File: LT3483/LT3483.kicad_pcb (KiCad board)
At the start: 2 copper layers, 19.8 x 40.1 mm, 15 parts

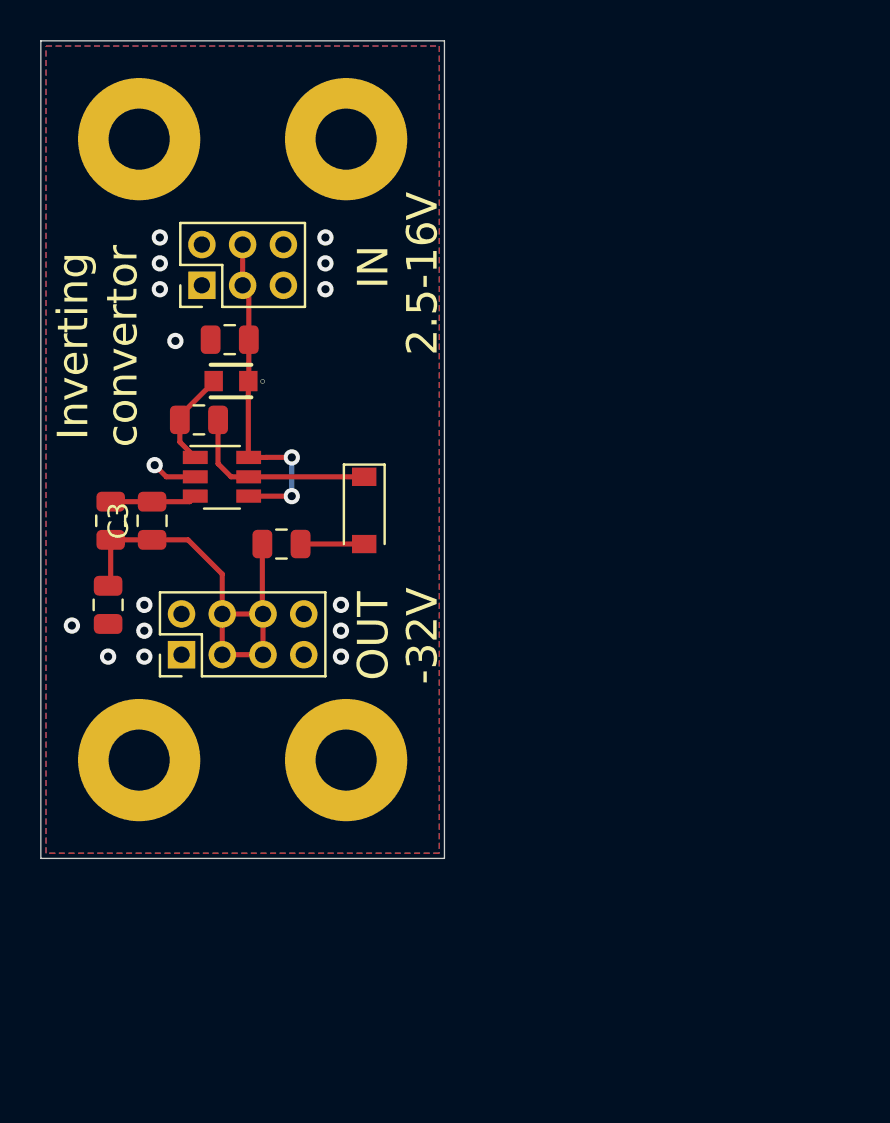
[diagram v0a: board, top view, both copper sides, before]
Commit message: Update
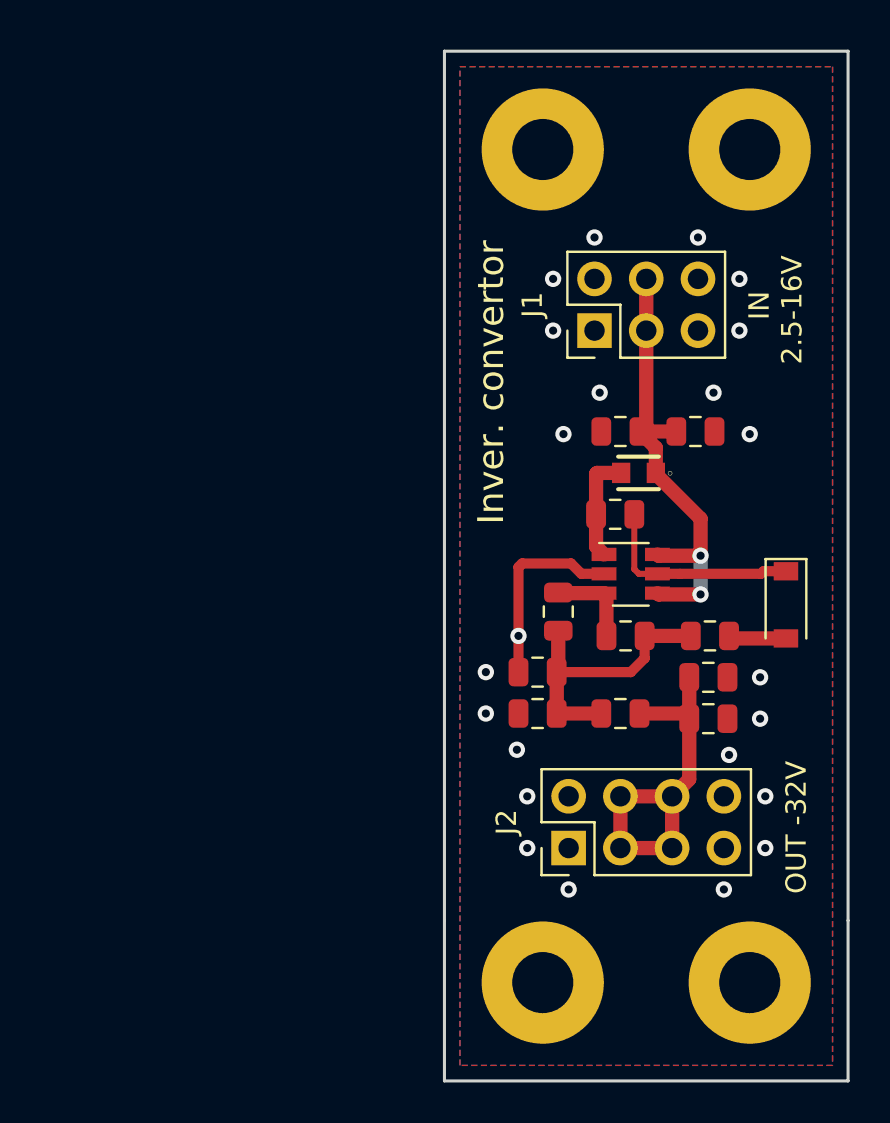
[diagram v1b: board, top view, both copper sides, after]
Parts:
- removed the ? at (155.0, 116.2)
- removed the ? at (157.4, 102.8)
- removed the ? at (151.4, 113.8)
- removed the ? at (156.0, 98.1)
- removed the ? at (157.4, 100.8)
- removed the ? at (155.8, 104.7)
- removed the ? at (159.9, 110.8)
- removed the ? at (151.5, 109.7)
- removed the ? at (157.0, 107.5)
- added C1: 4.7uF/30V, Capacitor_SMD:C_0805_2012Metric, F.Cu at (176.5, 105.3)
- added C2: 100nF/30V, Capacitor_SMD:C_0805_2012Metric, F.Cu at (180.2, 105.3)
- added C4: 5pF/50V, Capacitor_SMD:C_0805_2012Metric, F.Cu at (173.5, 114.1)
- added C5: 1uF/50V, Capacitor_SMD:C_0805_2012Metric, F.Cu at (172.5, 117.1)
- added C6: 100nF, Capacitor_SMD:C_0805_2012Metric, F.Cu at (172.5, 119.1)
- added C7: 100nF, Capacitor_SMD:C_0805_2012Metric, F.Cu at (180.8, 117.3)
- added C8: , Capacitor_SMD:C_0805_2012Metric, F.Cu at (180.8, 119.4)
- added J1: J1, Connector_PinHeader_2.54mm:PinHeader_2x03_P2.54mm_Vertical, F.Cu at (175.3, 100.3)
- added J2: J2, Connector_PinHeader_2.54mm:PinHeader_2x04_P2.54mm_Vertical, F.Cu at (174.0, 125.7)
- added L1: LQH2MCN100K02L, digikey-footprints:LQH2MCN100K02L, F.Cu at (177.4, 107.3)
- added R1: 39R, Resistor_SMD:R_0805_2012Metric, F.Cu at (180.9, 115.3)
- added R2: 3.2M, Resistor_SMD:R_0805_2012Metric, F.Cu at (176.8, 115.3)
- added R3: 100R, Resistor_SMD:R_0805_2012Metric, F.Cu at (176.5, 119.1)
- added U1: LT3483, Package_TO_SOT_SMD:TSOT-23-6, F.Cu at (177.0, 112.3)
- C3: value 5pF/50V -> 0.1uF/50V
- moved C3 22.7 mm to (176.3, 109.3), turned to 0 degrees
- moved ? 22.6 mm to (172.7, 132.3)
- moved ? 22.6 mm to (182.9, 132.3)
- moved D1 21.2 mm to (184.7, 113.8)
- moved ? 19.8 mm to (172.7, 91.4)
- moved ? 19.8 mm to (182.9, 91.4)
- gave numbers to parts that had none: 1
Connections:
- D1 pad 1: Net-(C2-Pad2) -> Net-(C3-Pad2)
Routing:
- net Net-(C7-Pad1): track 0.00 -> 18.9 mm
- net Net-(C3-Pad1): track 21.9 -> 5.37 mm
- net Net-(C4-Pad1): track 0.00 -> 14.2 mm
- net Net-(C2-Pad2): track 9.59 -> 0.00 mm
- net GND: track 2.23 -> 9.64 mm, vias 16 -> 23
- net Net-(C1-Pad2): track 16.7 -> 23.0 mm
- net Net-(C3-Pad2): track 4.26 -> 10.3 mm
- net Net-(C2-Pad1): track 4.75 -> 0.00 mm
- net Net-(C4-Pad2): track 0.00 -> 4.41 mm
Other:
- board size 19.8 x 40.1 mm -> 19.8 x 50.5 mm
- net class C1-Pad2 added: clearance 0.2, trace_width 0.5, via_dia 0.8, via_drill 0.4
- board text added: "Inver. convertor"
- board text removed: "Inverting convertor"
